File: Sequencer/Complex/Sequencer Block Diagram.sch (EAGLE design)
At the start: 2 parts, among them IC1 74386N

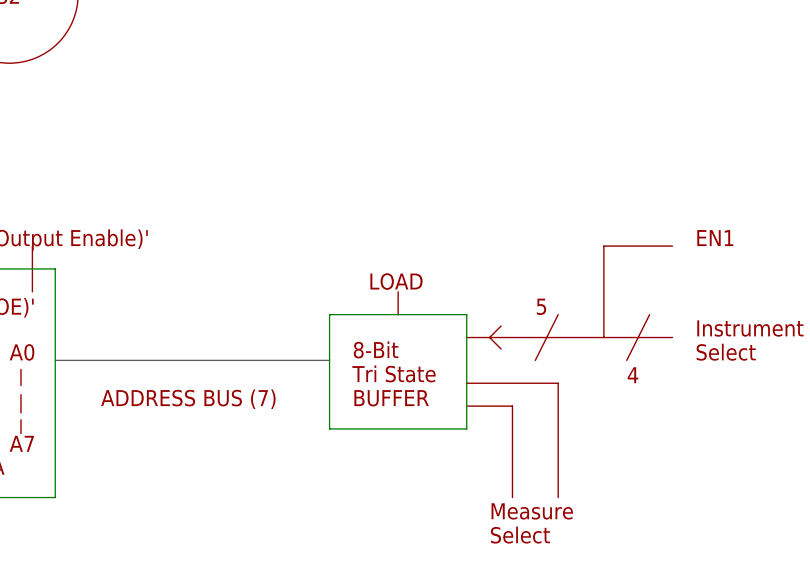
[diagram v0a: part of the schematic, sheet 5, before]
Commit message: k this should be good now
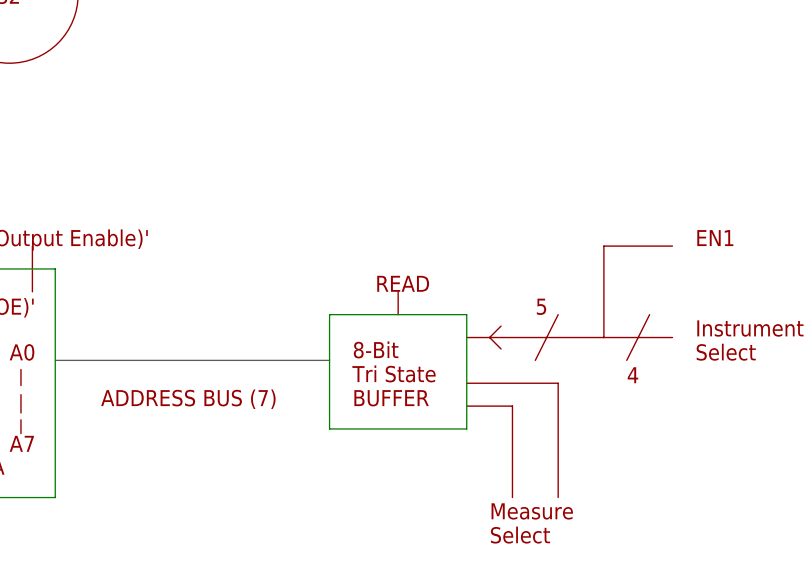
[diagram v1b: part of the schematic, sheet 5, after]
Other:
- note added: "READ"
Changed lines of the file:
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@@
 BUFFER</text>
 <wire x1="170.18" y1="99.06" x2="170.18" y2="101.6" width="0.1524" layer="94"/>
-<text x="166.878" y="101.854" size="1.778" layer="94">LOAD</text>
 <text x="40.64" y="91.44" size="1.778" layer="94">D-FF
 IN (0)</text>
@@
 <text x="40.64" y="71.12" size="1.778" layer="94">D-FF
 IN (1)</text>
+<text x="167.64" y="101.6" size="1.778" layer="94">READ</text>
 </plain>
 <instances>
